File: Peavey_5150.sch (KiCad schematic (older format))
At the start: 203 parts, among them J165 SEND, J166 RETURN, J2 Power, J3 OUTPUT, J37 INPUT FRONT, J39 INPUT REAR, J4 SWIM, J5 FOOTSWITCH, K1 G5V-2, K2 G5V-2, K3 G5V-2, K4 G5V-2, K5 G5V1, Q1 IRF840, Q2 BC847, Q3 BC847, Q4 BC847, SW2 Clean, SW3 Bright, SW4 FX_loop, U1 MP4462, U2 AMS1117-3.3, U3 STM8S003F3P, U4 TLP222A

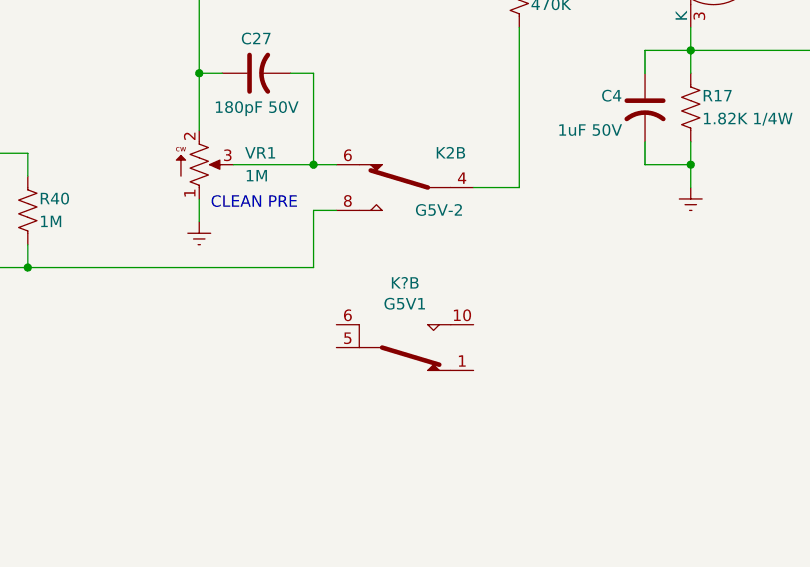
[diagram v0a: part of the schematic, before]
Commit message: Footprint update
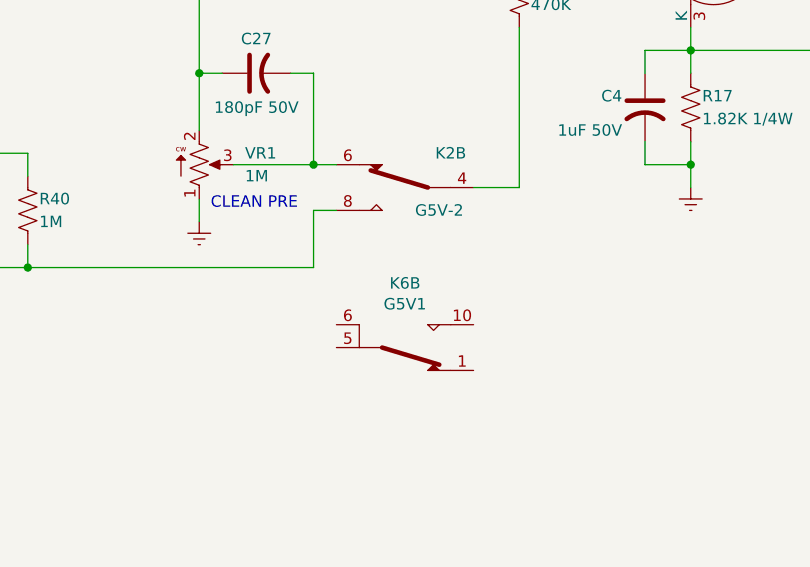
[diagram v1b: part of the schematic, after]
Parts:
- gave numbers to parts that had none: 1
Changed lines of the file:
@@
 NoConn ~ 18050 15500
 $Comp
-L Peavey_5150-rescue:G5V1-Relays-Peavey_5150-rescue K?
+L Peavey_5150-rescue:G5V1-Relays-Peavey_5150-rescue K6
 U 2 1 60063336
 P 8000 4800
-F 0 "K?" H 7950 4519 50  0000 C CNN
+F 0 "K6" H 7950 4519 50  0000 C CNN
 F 1 "G5V1" H 7950 4610 50  0000 C CNN
 F 2 "" H 8000 4800 50  0001 C CNN

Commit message: add relays
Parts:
- removed K2: G5V-2, symbol Peavey_5150-rescue:G5V-2-Relays-Peavey_5150-rescue
- added K2: G5V1, Peavey-EVH5150:Relay_SPDT_Omron_G5V-1, symbol Peavey_5150-rescue:G5V1-Relays-Peavey_5150-rescue
- added unit 1 of K6
- K1, K3, K4: footprint (none) -> Peavey-EVH5150:Relay_DPDT_Omron_G5V-2
- K5, K6: footprint (none) -> Peavey-EVH5150:Relay_SPDT_Omron_G5V-1
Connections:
- net at C52.1, R81.2, U4.3: now also K6.5, K6.6
- net at VR7.3: now also K6.10
- net at D7.1 (K), K1.1, R46.1: now also K2.2, K6.2
- net at D7.2 (A), K1.16, Q2.3 (C): now also K2.9, K6.9
- net at K6.1: now also VR6.3
- net at C27.2, VR1.3: now also K2.1
- net at R82.1: now also K2.5, K2.6
- net at C19.2, R40.1, VR2.3: now also K2.10
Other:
- note added: "12V 12.5mA"
- note added: "12V 41.7mA"
- moved on the sheet: K1A, K6B
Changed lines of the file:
@@
 EESchema Schematic File Version 4
-EELAYER 30 0
+LIBS:Peavey_5150-cache
+EELAYER 29 0
 EELAYER END
 $Descr A1 33110 23386
@@
 	22900 3250 23000 3250
 Wire Wire Line
-	23800 3500 23800 3150
+	23800 3500 23800 3250
 $Comp
 L Peavey_5150-rescue:R_POT_US_P-simple-Peavey_5150-rescue VR12
@@
 F 0 "K3" H 26650 3750 50  0000 C CNN
 F 1 "G5V-2" H 26700 3500 50  0000 C CNN
-F 2 "" H 26900 3650 50  0001 C CNN
+F 2 "Peavey-EVH5150:Relay_DPDT_Omron_G5V-2" H 26900 3650 50  0001 C CNN
 F 3 "" H 26900 3650 50  0001 C CNN
 	2    26900 3650
@@
 F 0 "K3" H 27505 15146 50  0000 L CNN
 F 1 "G5V-2" H 27505 15055 50  0000 L CNN
-F 2 "" H 27350 15100 50  0001 C CNN
+F 2 "Peavey-EVH5150:Relay_DPDT_Omron_G5V-2" H 27350 15100 50  0001 C CNN
 F 3 "" H 27350 15100 50  0001 C CNN
 	1    27350 15100
@@
 F 0 "K3" H 26650 5900 50  0000 C CNN
 F 1 "G5V-2" H 26700 5650 50  0000 C CNN
-F 2 "" H 26900 5800 50  0001 C CNN
+F 2 "Peavey-EVH5150:Relay_DPDT_Omron_G5V-2" H 26900 5800 50  0001 C CNN
 F 3 "" H 26900 5800 50  0001 C CNN
 	3    26900 5800
@@
 	23150 14700 22800 14700
 Wire Wire Line
-	22800 14700 22800 14800
+	22250 14700 22250 14800
 Connection ~ 23150 14700
 Wire Wire Line
 	23150 14700 23150 14800
 Wire Wire Line
-	22800 15400 22800 15500
+	22250 15400 22250 15500
 Wire Wire Line
-	22800 15500 23150 15500
+	22250 15500 22800 15500
 Connection ~ 23150 15500
 Wire Wire Line
@@
 Wire Wire Line
 	7650 4000 7550 4000
-$Comp
-L Peavey_5150-rescue:G5V-2-Relays-Peavey_5150-rescue K2
-U 2 1 61BF8E8B
-P 7900 4100
-F 0 "K2" H 7650 4250 50  0000 C CNN
-F 1 "G5V-2" H 7700 4000 50  0000 C CNN
-F 2 "" H 7900 4100 50  0001 C CNN
-F 3 "" H 7900 4100 50  0001 C CNN
-	2    7900 4100
-	-1   0    0    -1
-$EndComp
 Wire Wire Line
 	7050 4250 7050 4150
@@
 F 0 "K4" H 6350 2750 50  0000 C CNN
 F 1 "G5V-2" H 6400 2500 50  0000 C CNN
-F 2 "" H 6600 2600 50  0001 C CNN
+F 2 "Peavey-EVH5150:Relay_DPDT_Omron_G5V-2" H 6600 2600 50  0001 C CNN
 F 3 "" H 6600 2600 50  0001 C CNN
 	3    6600 2600
@@
 F 0 "K4" H 5850 2100 50  0000 C CNN
 F 1 "G5V-2" H 5900 1850 50  0000 C CNN
-F 2 "" H 6100 2000 50  0001 C CNN
+F 2 "Peavey-EVH5150:Relay_DPDT_Omron_G5V-2" H 6100 2000 50  0001 C CNN
 F 3 "" H 6100 2000 50  0001 C CNN
 	2    6100 2000
@@
 F 0 "K1" H 10600 5150 50  0000 C CNN
 F 1 "G5V-2" H 10650 4900 50  0000 C CNN
-F 2 "" H 10850 5000 50  0001 C CNN
+F 2 "Peavey-EVH5150:Relay_DPDT_Omron_G5V-2" H 10850 5000 50  0001 C CNN
 F 3 "" H 10850 5000 50  0001 C CNN
 	2    10850 5000
@@
 F 0 "K1" H 10600 4700 50  0000 C CNN
 F 1 "G5V-2" H 10650 4450 50  0000 C CNN
-F 2 "" H 10850 4550 50  0001 C CNN
+F 2 "Peavey-EVH5150:Relay_DPDT_Omron_G5V-2" H 10850 4550 50  0001 C CNN
 F 3 "" H 10850 4550 50  0001 C CNN
 	3    10850 4550
@@
 GNDPWR
 $Comp
-L Peavey_5150-rescue:G5V-2-Relays-Peavey_5150-rescue K2
-U 1 1 6AA3417A
-P 23150 15100
-F 0 "K2" H 22900 15150 50  0000 C CNN
-F 1 "G5V-2" H 22850 15050 50  0000 C CNN
-F 2 "" H 23150 15100 50  0001 C CNN
-F 3 "" H 23150 15100 50  0001 C CNN
-	1    23150 15100
-	-1   0    0    -1
-$EndComp
-$Comp
 L Peavey_5150-rescue:G5V-2-Relays-Peavey_5150-rescue K1
 U 1 1 6AA3618E
-P 22800 15100
-F 0 "K1" H 23050 15150 50  0000 C CNN
-F 1 "G5V-2" H 23100 15050 50  0000 C CNN
-F 2 "" H 22800 15100 50  0001 C CNN
-F 3 "" H 22800 15100 50  0001 C CNN
-	1    22800 15100
+P 22250 15100
+F 0 "K1" H 22500 15150 50  0000 C CNN
+F 1 "G5V-2" H 22550 15050 50  0000 C CNN
+F 2 "Peavey-EVH5150:Relay_DPDT_Omron_G5V-2" H 22250 15100 50  0001 C CNN
+F 3 "" H 22250 15100 50  0001 C CNN
+	1    22250 15100
 	-1   0    0    -1
 $EndComp
@@
 F 0 "K4" H 25200 15150 50  0000 C CNN
 F 1 "G5V-2" H 25250 15050 50  0000 C CNN
-F 2 "" H 24950 15100 50  0001 C CNN
+F 2 "Peavey-EVH5150:Relay_DPDT_Omron_G5V-2" H 24950 15100 50  0001 C CNN
 F 3 "" H 24950 15100 50  0001 C CNN
 	1    24950 15100
 	-1   0    0    -1
 $EndComp
-$Comp
-L Peavey_5150-rescue:G5V-2-Relays-Peavey_5150-rescue K2
-U 3 1 6AC21A8E
-P 23250 3150
-F 0 "K2" H 23000 3300 50  0000 C CNN
-F 1 "G5V-2" H 23050 3050 50  0000 C CNN
-F 2 "" H 23250 3150 50  0001 C CNN
-F 3 "" H 23250 3150 50  0001 C CNN
-	3    23250 3150
-	-1   0    0    -1
-$EndComp
 Wire Wire Line
 	23600 3150 23800 3150
@@
 F 0 "K5" H 7450 2869 50  0000 C CNN
 F 1 "G5V1" H 7450 2960 50  0000 C CNN
-F 2 "" H 7500 3150 50  0001 C CNN
+F 2 "Peavey-EVH5150:Relay_SPDT_Omron_G5V-1" H 7500 3150 50  0001 C CNN
 F 3 "" H 7500 3150 50  0001 C CNN
 	2    7500 3150
@@
 F 0 "K5" H 25645 15146 50  0000 R CNN
 F 1 "G5V1" H 25645 15055 50  0000 R CNN
-F 2 "" H 25800 15100 50  0001 C CNN
+F 2 "Peavey-EVH5150:Relay_SPDT_Omron_G5V-1" H 25800 15100 50  0001 C CNN
 F 3 "" H 25800 15100 50  0001 C CNN
 	1    25800 15100
@@
 L Peavey_5150-rescue:G5V1-Relays-Peavey_5150-rescue K6
 U 2 1 60063336
-P 8000 4800
-F 0 "K6" H 7950 4519 50  0000 C CNN
-F 1 "G5V1" H 7950 4610 50  0000 C CNN
-F 2 "" H 8000 4800 50  0001 C CNN
-F 3 "" H 8000 4800 50  0001 C CNN
-	2    8000 4800
-	1    0    0    1
+P 23250 3150
+F 0 "K6" H 23150 3400 50  0000 C CNN
+F 1 "G5V1" H 23150 3300 50  0000 C CNN
+F 2 "Peavey-EVH5150:Relay_SPDT_Omron_G5V-1" H 23250 3150 50  0001 C CNN
+F 3 "" H 23250 3150 50  0001 C CNN
+	2    23250 3150
+	-1   0    0    -1
 $EndComp
+$Comp
+L Peavey_5150-rescue:G5V1-Relays-Peavey_5150-rescue K2
+U 2 1 5FB967F2
+P 7900 4100
+F 0 "K2" H 7800 4350 50  0000 C CNN
+F 1 "G5V1" H 7800 4250 50  0000 C CNN
+F 2 "Peavey-EVH5150:Relay_SPDT_Omron_G5V-1" H 7900 4100 50  0001 C CNN
+F 3 "" H 7900 4100 50  0001 C CNN
+	2    7900 4100
+	-1   0    0    -1
+$EndComp
+Wire Wire Line
+	8250 4200 8450 4200
+Wire Wire Line
+	8450 4200 8450 4100
+Connection ~ 8450 4100
+Wire Wire Line
+	23600 3250 23800 3250
+Connection ~ 23800 3250
+Wire Wire Line
+	23800 3250 23800 3150
+$Comp
+L Peavey_5150-rescue:G5V1-Relays-Peavey_5150-rescue K2
+U 1 1 5FCD7242
+P 22800 15100
+F 0 "K2" H 22645 15146 50  0000 R CNN
+F 1 "G5V1" H 22645 15055 50  0000 R CNN
+F 2 "Peavey-EVH5150:Relay_SPDT_Omron_G5V-1" H 22800 15100 50  0001 C CNN
+F 3 "" H 22800 15100 50  0001 C CNN
+	1    22800 15100
+	1    0    0    -1
+$EndComp
+$Comp
+L Peavey_5150-rescue:G5V1-Relays-Peavey_5150-rescue K6
+U 1 1 5FCD95C4
+P 23150 15100
+F 0 "K6" H 22995 15146 50  0000 R CNN
+F 1 "G5V1" H 22995 15055 50  0000 R CNN
+F 2 "Peavey-EVH5150:Relay_SPDT_Omron_G5V-1" H 23150 15100 50  0001 C CNN
+F 3 "" H 23150 15100 50  0001 C CNN
+	1    23150 15100
+	-1   0    0    -1
+$EndComp
+Wire Wire Line
+	22800 14800 22800 14700
+Connection ~ 22800 14700
+Wire Wire Line
+	22800 14700 22250 14700
+Wire Wire Line
+	22800 15400 22800 15500
+Connection ~ 22800 15500
+Wire Wire Line
+	22800 15500 23150 15500
+Text Notes 22300 15250 0    20   ~ 0
+12V 41.7mA
+Text Notes 23200 15250 0    20   ~ 0
+12V 12.5mA
+Text Notes 22850 15250 0    20   ~ 0
+12V 12.5mA
 $EndSCHEMATC
